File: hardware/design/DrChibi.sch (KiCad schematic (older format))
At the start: 20 parts, among them P2 PAD_SMD, P3 IN+, P4 IN-, X1 MINI-USB-SHIELD-32005-201

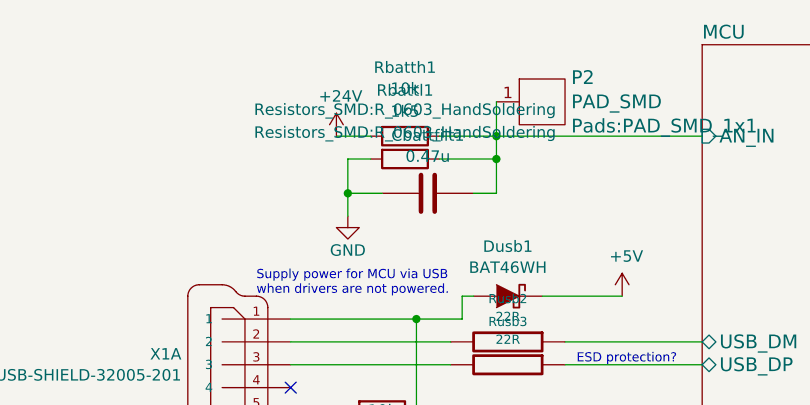
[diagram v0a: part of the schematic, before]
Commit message: TODO: Find appropriate routing to CPU
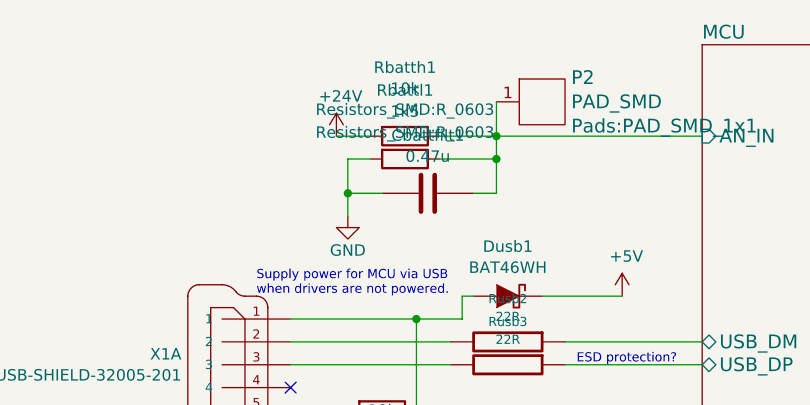
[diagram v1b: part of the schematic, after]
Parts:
- Rbatth1, Rbattl1: footprint Resistors_SMD:R_0603_HandSoldering -> Resistors_SMD:R_0603
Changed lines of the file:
@@
 F 0 "Rbatth1" V 1550 1000 50  0000 C CNN
 F 1 "10k" V 1642 1000 50  0000 C CNN
-F 2 "Resistors_SMD:R_0603_HandSoldering" V 1734 1000 50  0000 C CNN
+F 2 "Resistors_SMD:R_0603" V 1734 1000 50  0000 C CNN
 F 3 "" H 1850 1000 50  0000 C CNN
 	1    1850 1000
@@
 F 0 "Rbattl1" V 1550 1100 50  0000 C CNN
 F 1 "1k5" V 1642 1100 50  0000 C CNN
-F 2 "Resistors_SMD:R_0603_HandSoldering" V 1734 1100 50  0000 C CNN
+F 2 "Resistors_SMD:R_0603" V 1734 1100 50  0000 C CNN
 F 3 "" H 1850 1100 50  0000 C CNN
 	1    1850 1100

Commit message: TODO next: Rearrangement and routing of the analog inputs.
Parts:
- CONN1: footprint Socket_Strips:Socket_Strip_Straight_2x06 -> Pads:Pin_Header_Straight_2x06_Pitch1.27mm
- X1: footprint CRF1:con-cypressindustries-32005-201 -> Pads:MICRO-B_USB
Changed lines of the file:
@@
 F 0 "X1" H 1428 2046 50  0000 L CNN
 F 1 "MINI-USB-SHIELD-32005-201" H 1428 1954 50  0000 L CNN
-F 2 "CRF1:con-cypressindustries-32005-201" H 1150 2150 50  0001 C CNN
+F 2 "Pads:MICRO-B_USB" H 1150 2150 50  0001 C CNN
 F 3 "" H 1150 2000 60  0001 C CNN
 	1    1150 2000
@@
 F 0 "CONN1" H 1100 4908 50  0000 C CNN
 F 1 "MultiPort" H 1100 4816 50  0000 C CNN
-F 2 "Socket_Strips:Socket_Strip_Straight_2x06" H 1100 4724 50  0000 C CNN
+F 2 "Pads:Pin_Header_Straight_2x06_Pitch1.27mm" H 1100 4724 50  0000 C CNN
 F 3 "" H 1100 3150 50  0000 C CNN
 	1    1100 4350
